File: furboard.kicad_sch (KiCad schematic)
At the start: 25 parts, among them J1 USB_C_Receptacle_USB2.0_14P, U1 RP2040, U2 NCP1117-3.3_SOT223, Y1 12 MHz

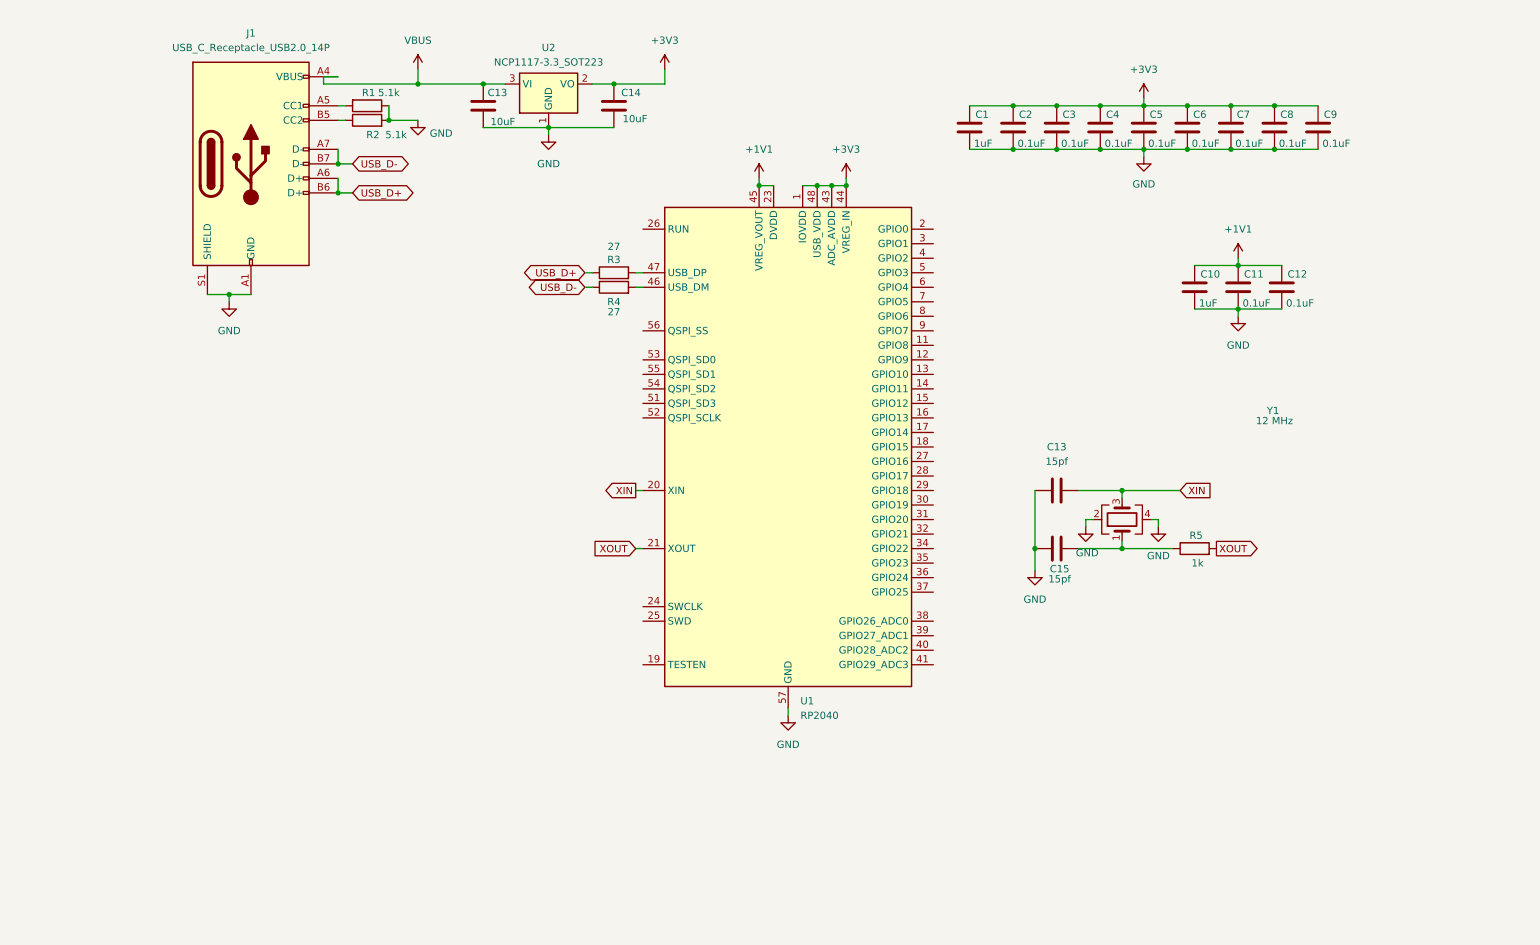
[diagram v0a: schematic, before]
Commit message: Update the sch to be more organized, also started adding flash storage
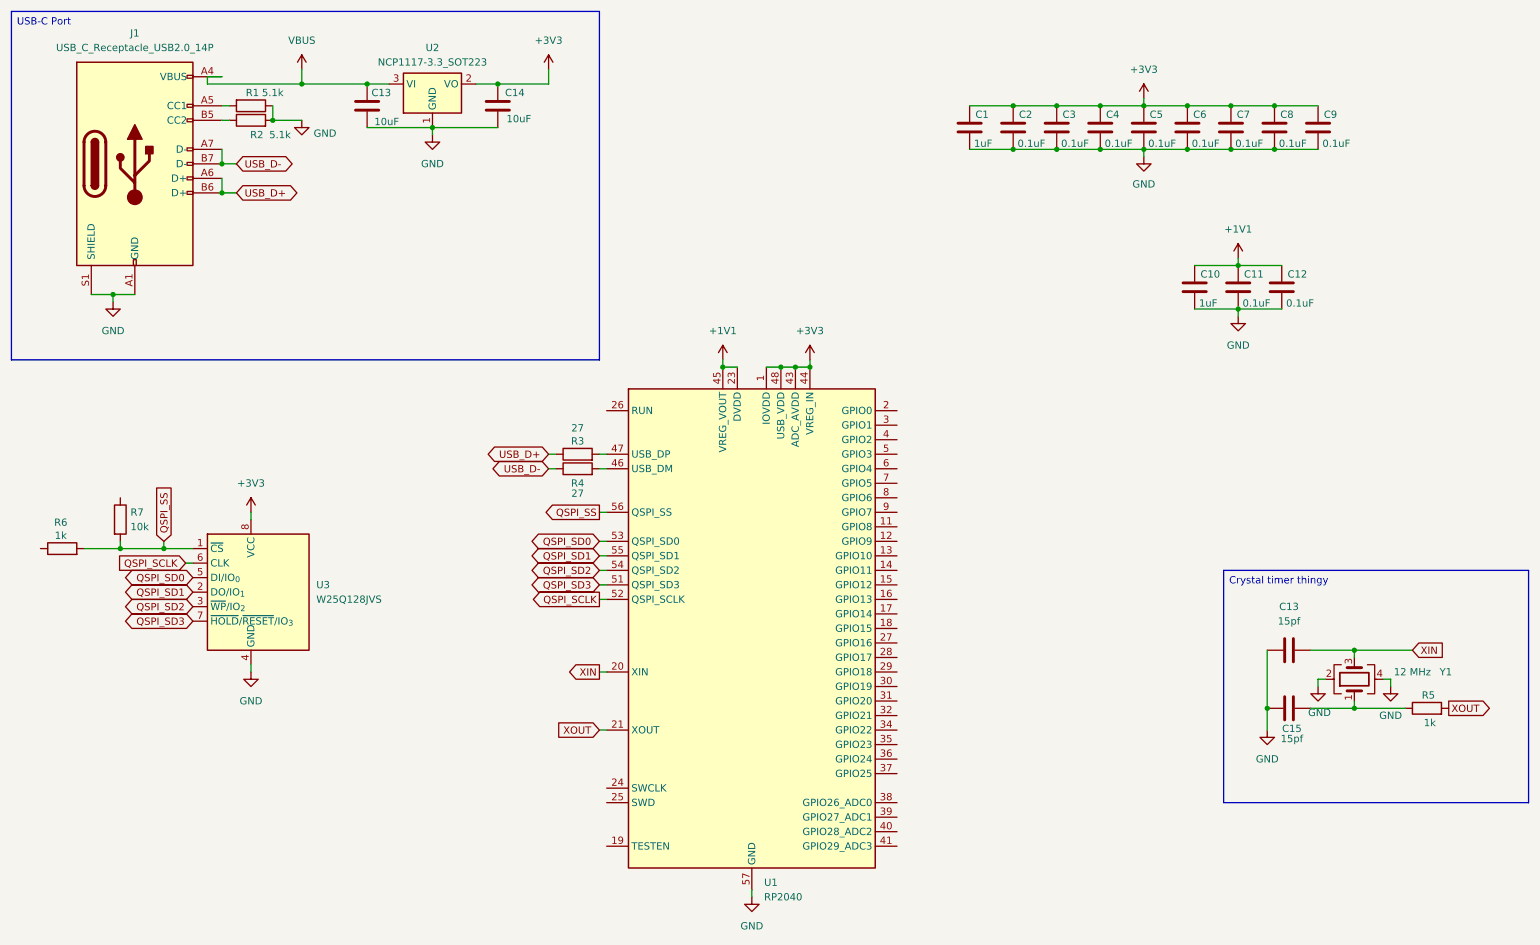
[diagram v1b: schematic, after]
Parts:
- added R6: 1k, symbol Device:R
- added R7: 10k, symbol Device:R
- added U3: W25Q128JVS, Package_SO:SOIC-8_5.3x5.3mm_P1.27mm, symbol Memory_Flash:W25Q128JVS
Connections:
- net +3V3: now also U3.8 (VCC)
- net GND: now also U3.4 (GND)
- net QSPI_SD3: now reaches U1.51 (QSPI_SD3)
- net QSPI_SD3: now also U3.7 (~{HOLD}/~{RESET}/IO_{3})
- net QSPI_SCLK: now reaches U1.52 (QSPI_SCLK)
- net QSPI_SCLK: now also U3.6 (CLK)
- net QSPI_SD0: now reaches U1.53 (QSPI_SD0)
- net QSPI_SD0: now also U3.5 (DI/IO_{0})
- net QSPI_SD2: now reaches U1.54 (QSPI_SD2)
- net QSPI_SD2: now also U3.3 (~{WP}/IO_{2})
- net QSPI_SD1: now reaches U1.55 (QSPI_SD1)
- net QSPI_SD1: now also U3.2 (DO/IO_{1})
- net QSPI_SS: now reaches U1.56 (QSPI_SS)
- net QSPI_SS: now also R6.2, R7.2, U3.1 (~{CS})
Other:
- moved on the sheet: 10uF, C13, C14, C15, J1, R1, R2, R3, R4, R5, U1, U2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
